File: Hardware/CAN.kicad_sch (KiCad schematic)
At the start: 9 parts, among them U2 SN65HVD230

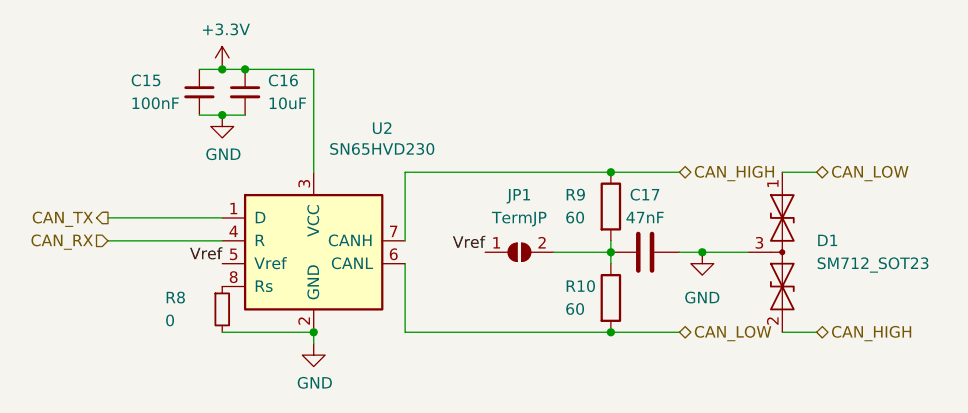
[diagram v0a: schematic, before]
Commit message: Revert "Merge remote-tracking branch 'refs/remotes/origin/main'"
This reverts commit c9a99cb72454eddb78504ad976151236a8d13e5c, reversing
changes made to 3cdb2e540a9938f01cf78ecb1078cc5742e66bb5.
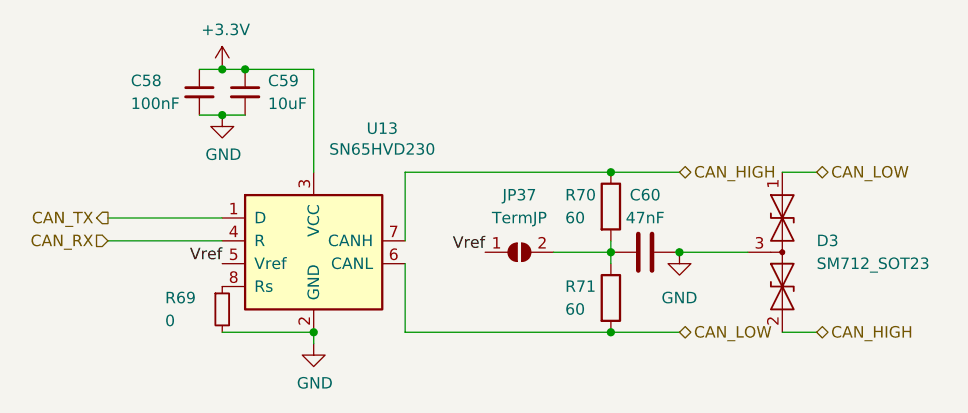
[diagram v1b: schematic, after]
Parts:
- C58: renamed from C15; footprint Capacitor_SMD:C_0402_1005Metric -> Capacitor_SMD:C_0603_1608Metric
- C59: renamed from C16; footprint Capacitor_SMD:C_0402_1005Metric -> Capacitor_SMD:C_0603_1608Metric
- renumbered C17 to C60, D1 to D3, JP1 to JP37, R8 to R69, R9 to R70, R10 to R71, U2 to U13

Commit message: Start of Kermit Mini
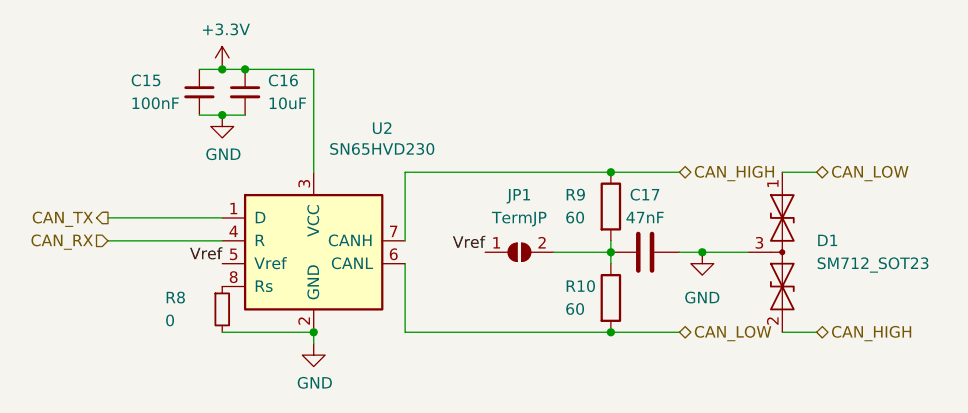
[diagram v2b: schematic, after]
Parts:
- C15: renamed from C58; footprint Capacitor_SMD:C_0603_1608Metric -> Capacitor_SMD:C_0402_1005Metric
- C16: renamed from C59; footprint Capacitor_SMD:C_0603_1608Metric -> Capacitor_SMD:C_0402_1005Metric
- renumbered C60 to C17, D3 to D1, JP37 to JP1, R71 to R10, R69 to R8, R70 to R9, U13 to U2
